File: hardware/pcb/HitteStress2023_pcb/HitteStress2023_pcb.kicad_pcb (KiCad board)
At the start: 2 copper layers, 152.5 x 101.9 mm, 9 parts, among them J1 Conn_01x02_Socket, J2 Conn_01x02_Socket, J3 SMA_conector_female, U1 MINIDCDCBOOST5V, U2 TTGO_T-Beam_T22_V1.1

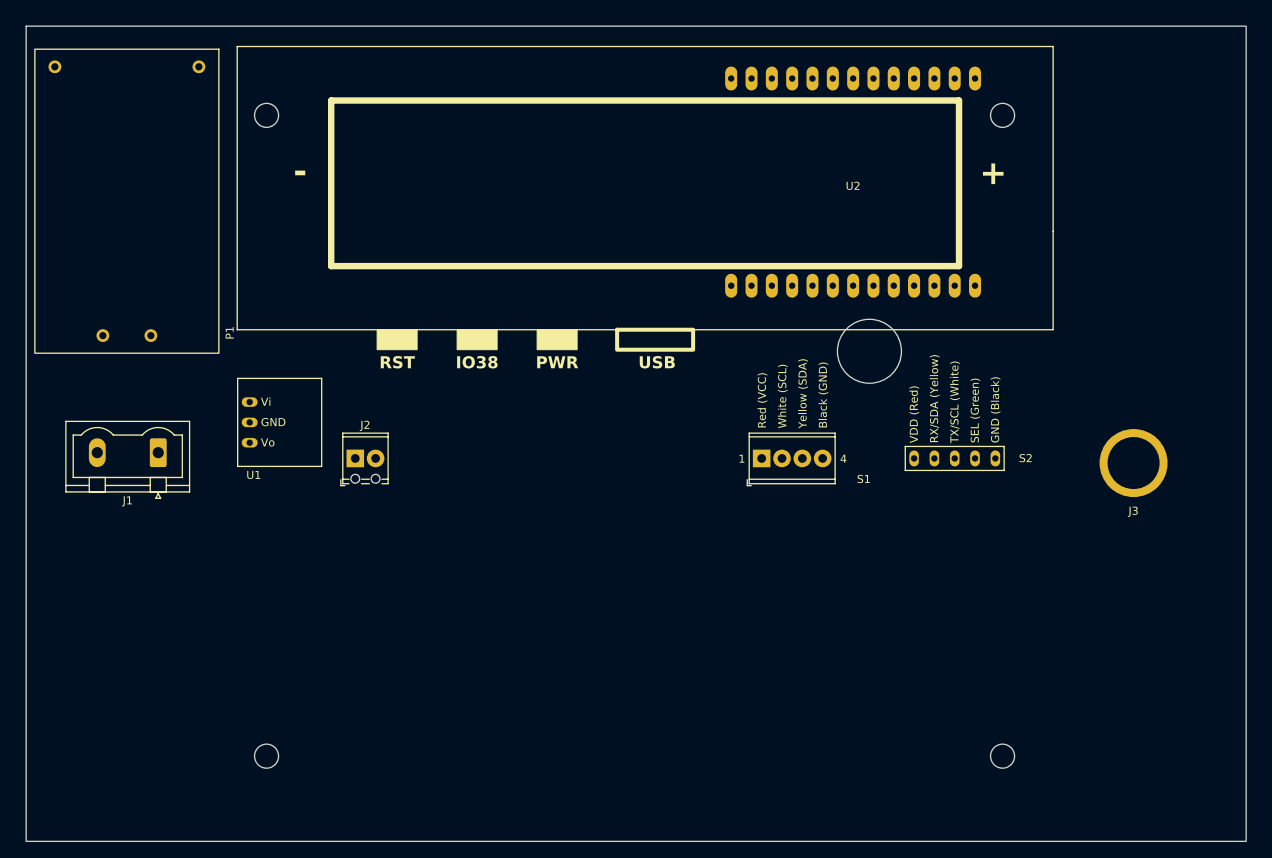
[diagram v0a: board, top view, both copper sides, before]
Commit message: Updates
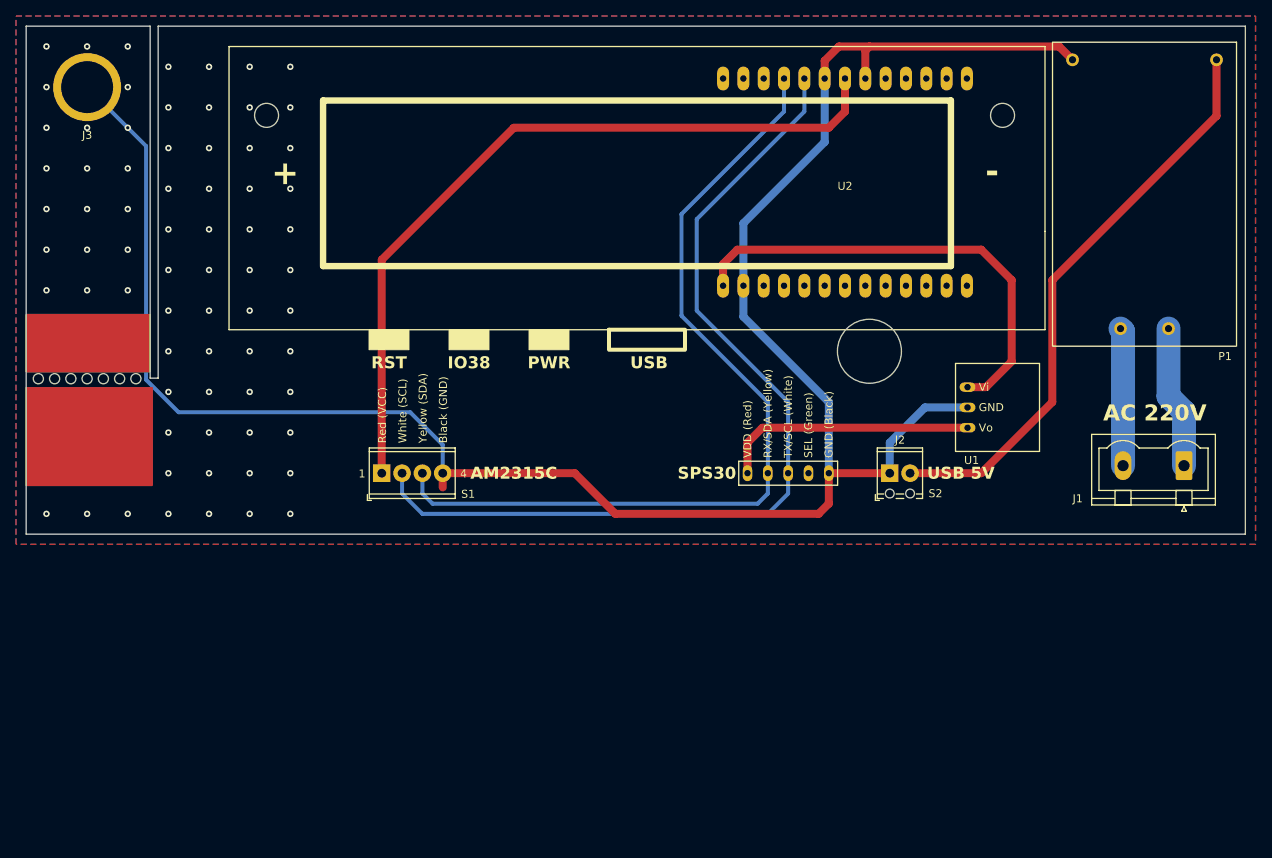
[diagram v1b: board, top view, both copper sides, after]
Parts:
- removed ?: , clipboard:8f7ff42e-40b4-4b4c-8b05-df8b6ae42a08
- U2: value TTGO_T-Beam_T22_V1.1 -> TTGO T-Beam T22 V1.1
- moved J3 139.0 mm to (86.4, 43.2)
- moved J1 128.2 mm to (223.5, 90.5)
- moved P1 127.2 mm to (207.0, 75.6)
- moved U1 89.7 mm to (196.4, 83.2)
- moved J2 66.8 mm to (186.7, 91.4)
- moved S1 47.5 mm to (123.3, 91.5)
- moved S2 20.9 mm to (174.0, 91.4)
- moved U2 1.02 mm to (206.1, 73.5)
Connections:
- J3 pad 1: unconnected-(J3-Pin_1-Pad1) -> /GND
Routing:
- net /GND: track 0.00 -> 259.9 mm, vias 0 -> 71
- net /SCL: track 0.00 -> 115.1 mm
- net /SDA: track 0.00 -> 108.4 mm
- net /3V3: track 0.00 -> 96.4 mm
- net /5V_I: track 0.00 -> 72.7 mm
- net /5V_U: track 0.00 -> 58.1 mm
- net /5V_SPS: track 0.00 -> 32.1 mm
- net Net-(J1-Pin_1): track 0.00 -> 17.9 mm
- net Net-(J1-Pin_2): track 0.00 -> 17.3 mm
- added copper zone on B.Cu, net /GND
- added copper zone on F.Cu, net /GND
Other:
- board size 152.5 x 101.9 mm -> 152.4 x 63.5 mm
- board text added: "AC 220V"
- board text added: "AM2315C"
- board text added: "SPS30"
- board text added: "USB 5V"
